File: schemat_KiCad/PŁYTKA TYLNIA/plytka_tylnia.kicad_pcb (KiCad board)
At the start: 2 copper layers, 113.5 x 70.2 mm, 36 parts, among them P1 USB_OTG, SW1 SPST

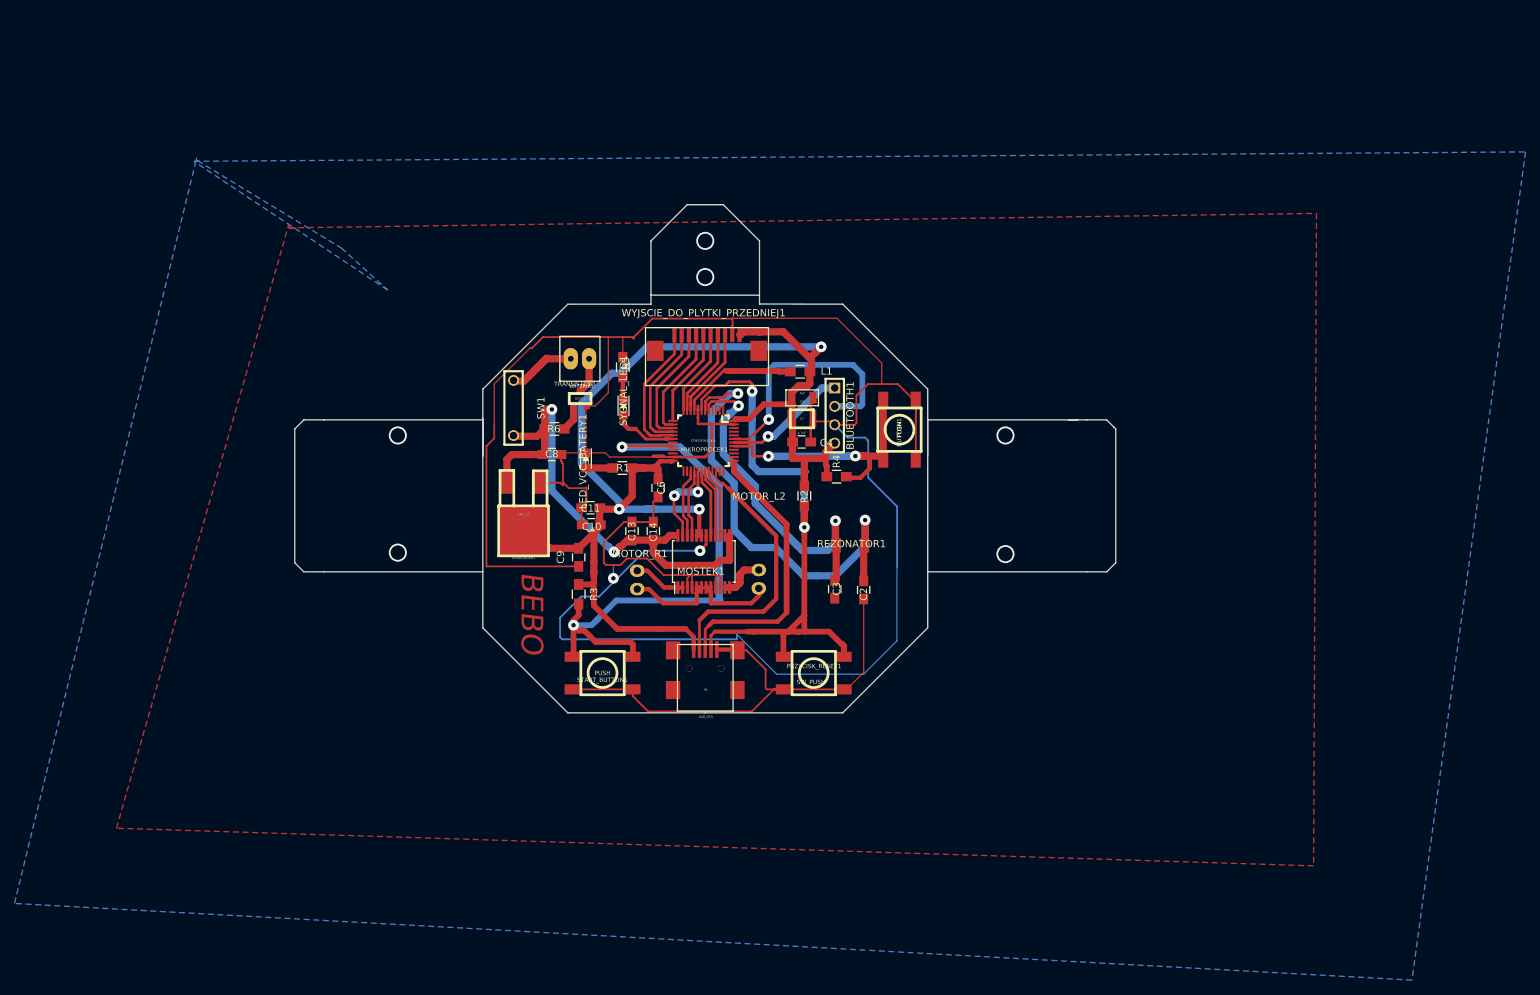
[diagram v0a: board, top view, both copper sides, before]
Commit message: tył do druku
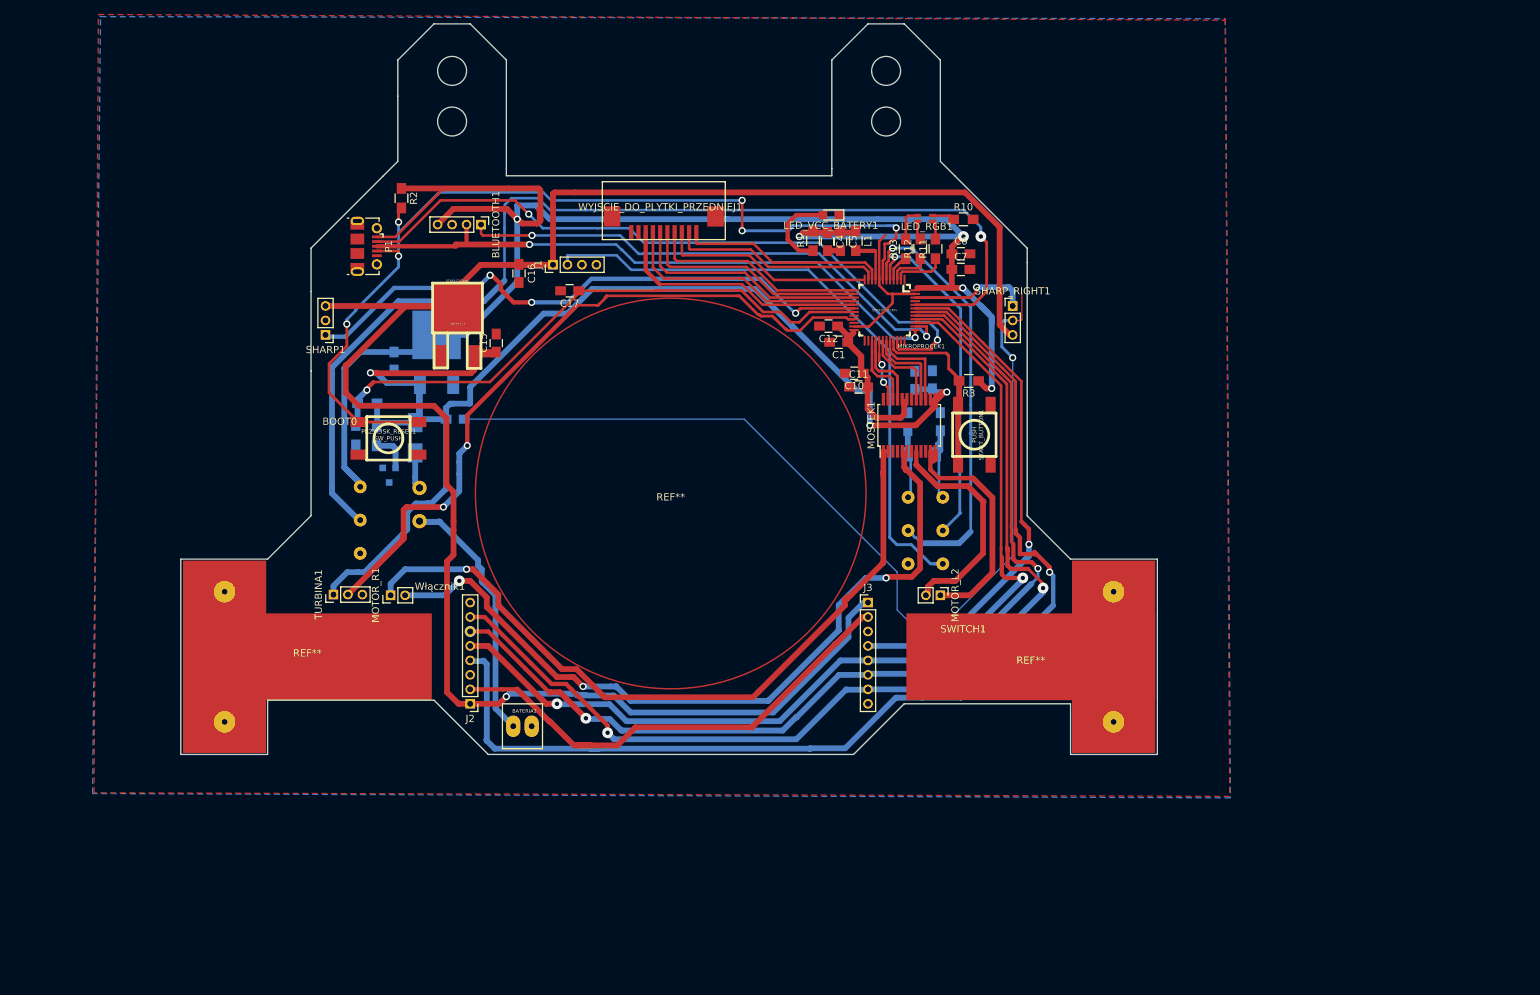
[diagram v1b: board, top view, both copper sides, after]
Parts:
- removed BUTTON1: PUSH, warsztatymisc:SW_06_SMD
- removed R4: 10k, Resistors_SMD:R_0805_HandSoldering
- removed R5: 200, Resistors_SMD:R_0805_HandSoldering
- removed SW1: SPST, warsztatymisc:dip_switch_1
- removed SYGNAL_LED1: LED_BLUE, LEDs:LED_0805
- added BOOT0: SWITCH, warsztaty:PRZEŁĄCZNIK_1x3, F.Cu at (94.8, 94.0)
- added Bezpiecznik1: Fuse ??, Fuse_Holders_and_Fuses:Fuse_SMD1206_HandSoldering, B.Cu at (102.4, 87.2)
- added C1: 4,7uF, Capacitors_SMD:C_0805_HandSoldering, F.Cu at (160.9, 74.0)
- added C12: 100nF, Capacitors_SMD:C_0805_HandSoldering, F.Cu at (159.5, 71.8)
- added C15: 10uF, Capacitors_SMD:C_0805_HandSoldering, F.Cu at (113.6, 74.1)
- added C16: 10uF, Capacitors_SMD:C_0805_HandSoldering, F.Cu at (116.8, 64.5)
- added C17: C, Capacitors_SMD:C_0805_HandSoldering, F.Cu at (123.8, 66.9)
- added J1: CONN_01X04, Pin_Headers:Pin_Header_Straight_1x04_Pitch2.00mm, F.Cu at (121.5, 63.3)
- added J2: PIN8, Pin_Headers:Pin_Header_Straight_1x08_Pitch2.00mm, F.Cu at (110.0, 124.0)
- added J3: PIN8, Pin_Headers:Pin_Header_Straight_1x08_Pitch2.00mm, F.Cu at (165.0, 110.0)
- added LED_RGB1: LED_CRGB, warsztaty:LED_RGB_0805, F.Cu at (172.9, 56.9)
- added R10: R, Resistors_SMD:R_0805_HandSoldering, F.Cu at (178.2, 57.0)
- added R11: R, Resistors_SMD:R_0805_HandSoldering, F.Cu at (174.3, 61.1)
- added R12: R, Resistors_SMD:R_0805_HandSoldering, F.Cu at (172.2, 61.1)
- added R13: R, Resistors_SMD:R_0805_HandSoldering, F.Cu at (170.2, 61.1)
- added R7: 51k, Resistors_SMD:R_0805_HandSoldering, B.Cu at (95.8, 82.4)
- added R8: 33k, Resistors_SMD:R_0805_HandSoldering, B.Cu at (94.2, 86.9)
- added REF**: Napęd_tunelowy, Napęd_tunelowy, F.Cu at (137.7, 94.9)
- added REF**: Silnik Pololu, warsztaty:Pololu_silnik, F.Cu at (187.5, 117.5)
- added REF**: Silnik Pololu, warsztaty:Pololu_silnik, F.Cu at (87.5, 117.5)
- added SHARP1: PIN3, Pin_Headers:Pin_Header_Straight_1x03_Pitch2.00mm, F.Cu at (90.0, 73.0)
- added SHARP_RIGHT1: PIN3, Pin_Headers:Pin_Header_Straight_1x03_Pitch2.00mm, F.Cu at (185.0, 69.0)
- added STABILIZATOR2: LM1117DT, warsztaty:LM1117_TO-252, F.Cu at (108.2, 75.9)
- added SWITCH1: Przełącznik_dźwigniowy_podwójny_On-On_MTS, warsztaty:PRZEŁĄCZNIK_2x3, F.Cu at (175.3, 104.7)
- added TURBINA1: PIN3, Pin_Headers:Pin_Header_Straight_1x03_Pitch2.00mm, F.Cu at (91.1, 108.9)
- added Włącznik1: switch, warsztaty:PRZEŁĄCZNIK_1x2, F.Cu at (103.0, 98.8)
- BATERIA1: footprint warsztatymisc:zl_zasilania -> misc:zl_zasilania
- BLUETOOTH1: footprint warsztatymisc:pin_array_4x1 -> Pin_Headers:Pin_Header_Straight_1x04_Pitch2.00mm
- C13, C14, C2, C3, C8, C9, R6, STABILIZATOR1: moved to B.Cu
- C5: footprint warsztatymisc:1206 -> Capacitors_SMD:C_0805_HandSoldering
- C7: footprint warsztatymisc:1210 -> Capacitors_SMD:C_0805_HandSoldering
- MIKROPROCEK1: footprint warsztatymisc:LQFP48 -> misc:LQFP48
- MOTOR_L2, MOTOR_R1: footprint warsztatymisc:silnik -> Pin_Headers:Pin_Header_Straight_1x02_Pitch2.00mm
- P1: footprint warsztatymisc:USB-MINI-B-SMD -> Connectors_USB:USB_Micro-B_Molex-105017-0001
- PRZYCISK_RESET1, START_BUTTON1: footprint warsztatymisc:SW_06_SMD -> misc:SW_06_SMD
- REZONATOR1: footprint warsztatymisc:Kwarc_SMD_Mini -> misc:Kwarc_SMD_Mini; moved to B.Cu
- TRANSISTOR1: footprint warsztatymisc:SOT23-3 -> misc:SOT23-3; moved to B.Cu
- WYJSCIE_DO_PLYTKI_PRZEDNIEJ1: footprint warsztatymisc:fpc_10_pin -> misc:fpc_10_pin
- moved P1 79.5 mm to (94.8, 60.8), turned to 270 degrees
- moved R2 69.3 mm to (100.5, 54.1)
- moved PRZYCISK_RESET1 67.2 mm to (98.7, 87.3)
- moved R3 61.5 mm to (178.9, 79.4), turned to 180 degrees
- moved START_BUTTON1 61.1 mm to (179.7, 86.8), turned to 270 degrees
- moved BLUETOOTH1 55.6 mm to (111.5, 57.8)
- moved C6 52.9 mm to (177.8, 61.8), turned to 0 degrees
- moved BATERIA1 51.4 mm to (120.0, 124.0)
- moved LED_VCC_BATERY1 47.9 mm to (159.9, 56.4), turned to 180 degrees
- moved C13 44.3 mm to (171.5, 79.3)
- moved C14 43.9 mm to (173.9, 79.2)
- moved C10 42.0 mm to (163.1, 78.3)
- moved R1 41.0 mm to (157.4, 60.0), turned to 90 degrees
- moved C11 40.6 mm to (163.7, 80.2)
- moved C9 37.3 mm to (99.5, 76.6)
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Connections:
- BATERIA1 pad 1: Net-(BATERIA1-Pad1) -> GND
- BLUETOOTH1 pad 2: /USART_TX -> /SWCLK
- C2 pad 1: Net-(C3-Pad1) -> Net-(C2-Pad1)
- C3 pad 1: Net-(C2-Pad1) -> Net-(C3-Pad1)
- MIKROPROCEK1 pad 18: Net-(MIKROPROCEK1-Pad45) -> /SHARP_LEFT
- MIKROPROCEK1 pad 19: (no net) -> /LIPOL_POMIAR
- MIKROPROCEK1 pad 2: (no net) -> /LED_R
- MIKROPROCEK1 pad 20: Net-(MIKROPROCEK1-Pad20) -> (no net)
- MIKROPROCEK1 pad 21: (no net) -> /TURBINA_PWM
- MIKROPROCEK1 pad 3: (no net) -> /LED_G
- MIKROPROCEK1 pad 33: (no net) -> Net-(MIKROPROCEK1-Pad33)
- MIKROPROCEK1 pad 38: (no net) -> /USART_RX
- MIKROPROCEK1 pad 39: (no net) -> /SPI1_CLK
- MIKROPROCEK1 pad 4: (no net) -> /LED_B
- MIKROPROCEK1 pad 40: (no net) -> /SPI1_MISO
- MIKROPROCEK1 pad 41: Net-(BUTTON1-Pad2) -> /SPI1_MOSI
- MIKROPROCEK1 pad 42: /USART_RX -> /SPI1_SS1
- MIKROPROCEK1 pad 43: /USART_TX -> /SPI1_SS2
- MIKROPROCEK1 pad 44: (no net) -> /BOOT0
- MIKROPROCEK1 pad 46: (no net) -> /SHARP_RIGHT
- MIKROPROCEK1 pad 5: Net-(C2-Pad1) -> /OSC_IN
- MIKROPROCEK1 pad 6: Net-(C3-Pad1) -> (no net)
- R3 pad 2: Net-(MIKROPROCEK1-Pad20) -> Net-(MIKROPROCEK1-Pad33)
- R6 pad 1: Net-(C8-Pad1) -> /BATERIA
- R6 pad 2: /BATERIA -> Net-(R6-Pad2)
- REZONATOR1 pad 1: Net-(C2-Pad1) -> Net-(C3-Pad1)
- REZONATOR1 pad 2: Net-(C3-Pad1) -> Net-(C2-Pad1)
- START_BUTTON1 pad 2: Net-(MIKROPROCEK1-Pad20) -> Net-(MIKROPROCEK1-Pad33)
- TRANSISTOR1 pad 1: Net-(C8-Pad1) -> GND
- TRANSISTOR1 pad 2: GND -> Net-(R6-Pad2)
- TRANSISTOR1 pad 3: Net-(BATERIA1-Pad1) -> GND
- WYJSCIE_DO_PLYTKI_PRZEDNIEJ1 pad 1: /T8 -> /T1
- WYJSCIE_DO_PLYTKI_PRZEDNIEJ1 pad 2: /T7 -> /T2
- WYJSCIE_DO_PLYTKI_PRZEDNIEJ1 pad 3: /T6 -> /T3
- WYJSCIE_DO_PLYTKI_PRZEDNIEJ1 pad 4: /T5 -> /T4
- WYJSCIE_DO_PLYTKI_PRZEDNIEJ1 pad 5: /T4 -> /T5
- WYJSCIE_DO_PLYTKI_PRZEDNIEJ1 pad 6: /T3 -> /T6
- WYJSCIE_DO_PLYTKI_PRZEDNIEJ1 pad 7: /T2 -> /T7
- WYJSCIE_DO_PLYTKI_PRZEDNIEJ1 pad 8: /T1 -> /T8
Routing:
- net /5V: track 0.00 -> 333.5 mm, vias 0 -> 1
- net GND: track 444.1 -> 156.8 mm, vias 2 -> 1
- net /SPI1_SS1: track 0.00 -> 227.1 mm, vias 0 -> 1
- net VCC: track 205.5 -> 426.5 mm, vias 3 -> 5
- net /SPI1_MISO: track 0.00 -> 186.0 mm, vias 0 -> 2
- net /SPI1_CLK: track 0.00 -> 160.4 mm, vias 0 -> 2
- net /BOOT0: track 0.00 -> 150.0 mm, vias 0 -> 1
- net /SPI1_MOSI: track 0.00 -> 148.8 mm, vias 0 -> 3
- net /BATERIA: track 71.2 -> 219.8 mm, vias 2 -> 3
- net Net-(MOSTEK1-Pad1): track 7.59 -> 135.5 mm, vias 0 -> 1
- net Net-(MOSTEK1-Pad5): track 12.9 -> 128.3 mm, vias 0 -> 3
- net /TURBINA_PWM: track 0.00 -> 99.3 mm, vias 0 -> 2
- net /TRIG: track 0.00 -> 87.2 mm
- net /SHARP_LEFT: track 0.00 -> 84.2 mm, vias 0 -> 4
- net /LIPOL_POMIAR: track 0.00 -> 82.6 mm, vias 0 -> 1
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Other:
- board size 113.5 x 70.2 mm -> 135 x 101 mm
- board text added: "L.F. ANT"
- board text removed: "BEBO"
